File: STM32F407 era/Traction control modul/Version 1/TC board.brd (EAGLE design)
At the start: 79.7 x 100 mm, 70 parts, among them IC1 74HC14D, IC2 lm2575, IC3 74AC08D, IC5 REG1117, IC6 74AC14D, J1 CON1, U1 MAX13052ESA+, U2 MAX232AEWE+, U3 MAX531AESD+, X1 057-006-1

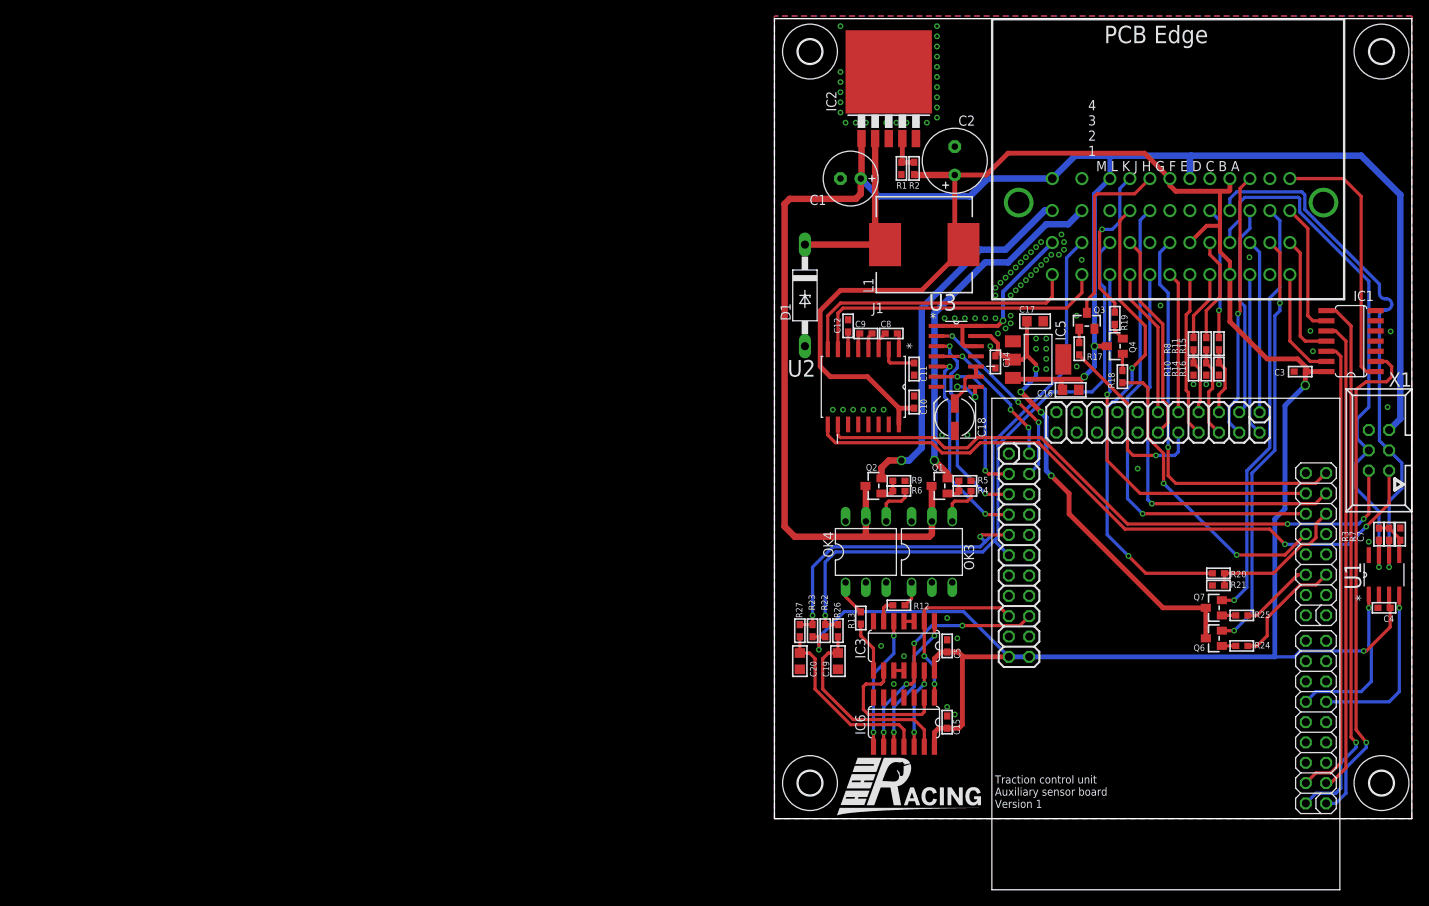
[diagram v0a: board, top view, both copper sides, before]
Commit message: started work on TC V2
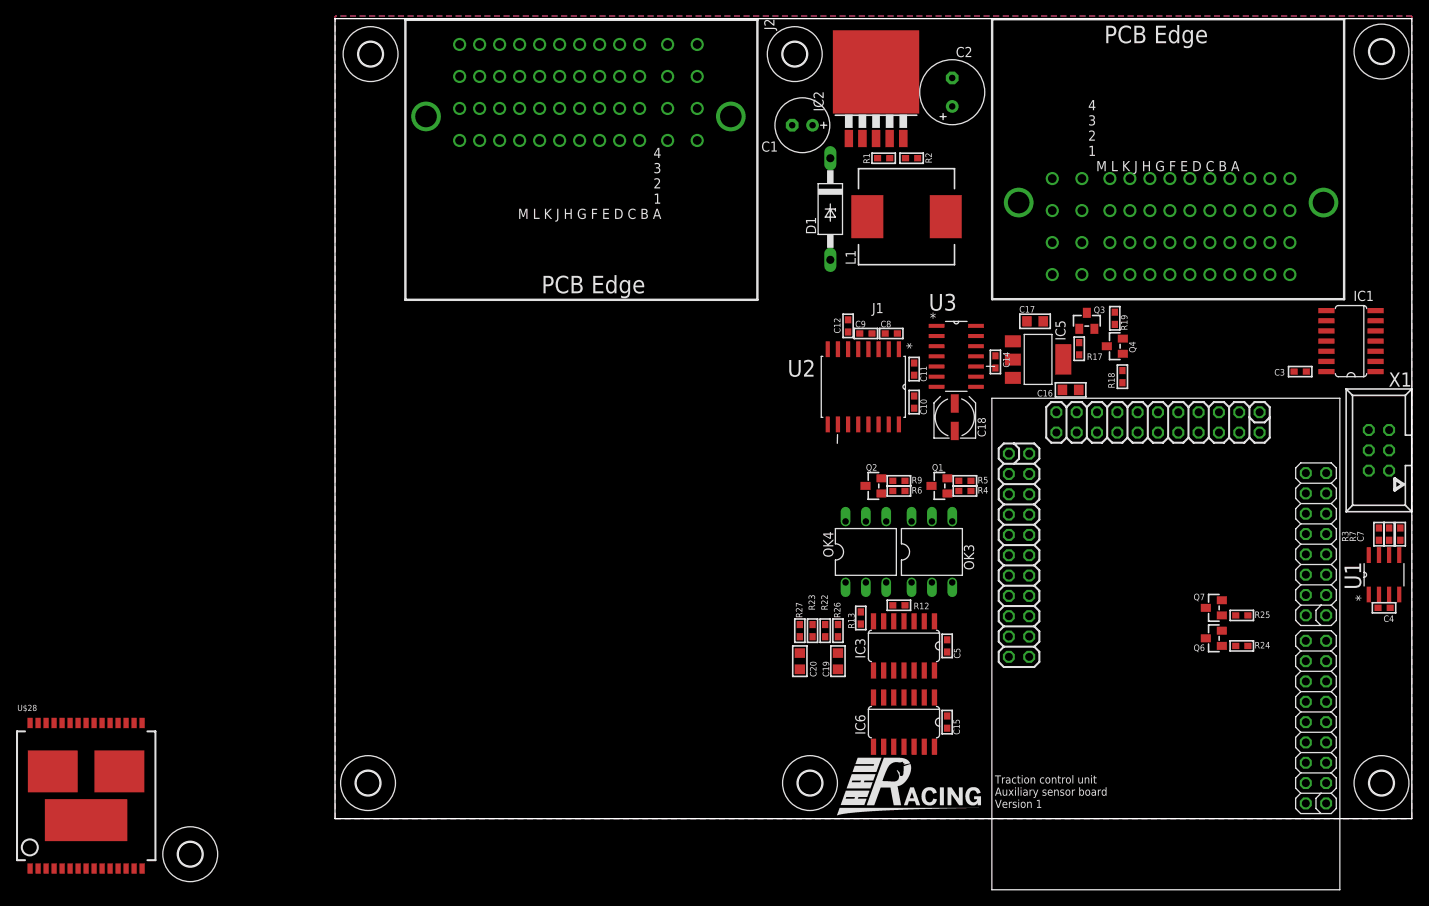
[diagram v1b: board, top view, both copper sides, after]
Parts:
- removed R10, R14, R16, R20: 178, microbuilder:_0603
- removed R11, R15, R21, R8: 604, microbuilder:_0603
- added H5, H6, H7: MOUNT-HOLE3.0, holes:3,0
- added J2: CON1, unicorn_v2:AUTOCONNECTOR
- added U$28: VNH2SP30, SparkFun-PowerIC:VNH2SP30
- moved D1 11.3 mm to (153.0, 92.4)
- moved C1 8.99 mm to (149.5, 102.9)
- moved C2 8.58 mm to (168.3, 107.0)
- moved L1 4.14 mm to (162.6, 91.4)
- moved R1 2.56 mm to (159.7, 98.7), turned to 0 degrees
- moved H2 1.93 mm to (148.6, 111.8)
- moved IC2 1.59 mm to (158.8, 107.0)
- moved R2 1.31 mm to (163.2, 98.7), turned to 180 degrees
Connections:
- net BITE: no longer R15.2
- net BITEO: no longer R15.1, R16.2
- net FUEL-RECIEVE: no longer R21.2
- net FUEL-RECIEVEI: no longer R20.2, R21.1
- net GND: no longer R10.1, R14.1, R16.1, R20.1
- net GSENS: no longer R8.2
- net GSENSO: no longer R10.2, R8.1
- net YAW: no longer R11.2
- net YAWO: no longer R11.1, R14.2
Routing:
- net 3.3V: track 284.1 -> 0.00 mm, vias 3 -> 0
- net 12V: track 235.5 -> 0.00 mm, vias 2 -> 0
- net COMRX: track 84.4 -> 0.00 mm, vias 2 -> 0
- net DIRBSENSE: track 80.9 -> 0.00 mm, vias 1 -> 0
- net COMTX: track 79.3 -> 0.00 mm, vias 2 -> 0
- net DIRASENSE: track 78.7 -> 0.00 mm, vias 2 -> 0
- net CANL: track 69.4 -> 0.00 mm, vias 1 -> 0
- net CANH: track 68.4 -> 0.00 mm, vias 1 -> 0
- net RPM2: track 67.9 -> 0.00 mm, vias 1 -> 0
- net RPM1: track 63.5 -> 0.00 mm, vias 1 -> 0
- net 5.0V: track 62.7 -> 0.00 mm, vias 4 -> 0
- net VTEMP2: track 60.2 -> 0.00 mm, vias 1 -> 0
- net FUEL-RECIEVE: track 59.6 -> 0.00 mm, vias 2 -> 0
- net RPM3: track 59.6 -> 0.00 mm
- net RPM4: track 58.3 -> 0.00 mm
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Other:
- board size 79.7 x 100 mm -> 134.6 x 100 mm

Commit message: Revert "started work on TC V2"
This reverts commit da86986705d51cbc4691d6d7bad1c5aae1ca4806.
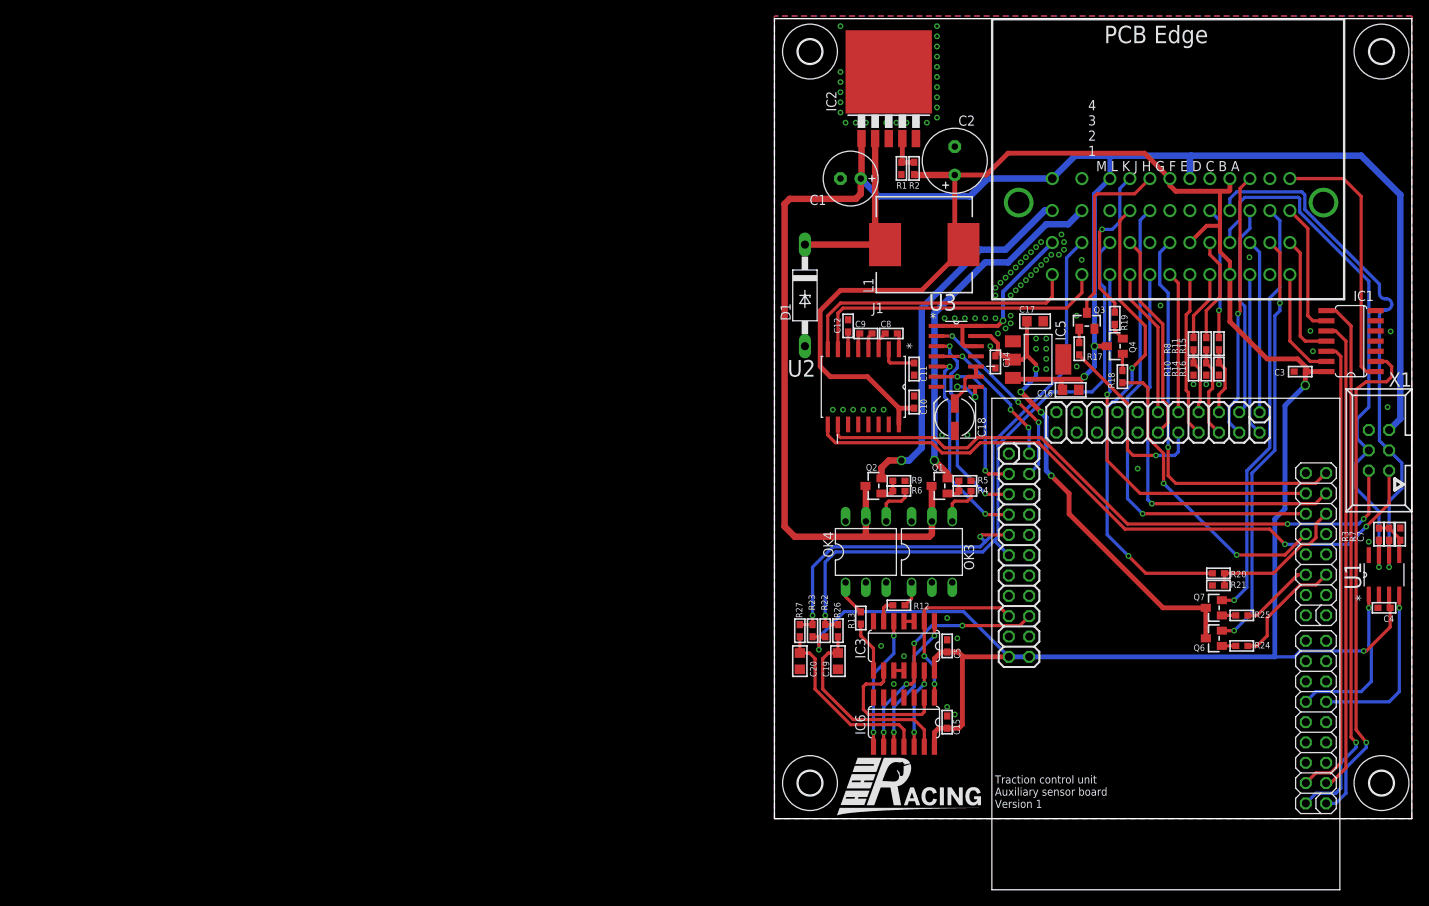
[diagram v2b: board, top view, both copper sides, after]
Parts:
- removed H5, H6, H7: MOUNT-HOLE3.0, holes:3,0
- removed J2: CON1, unicorn_v2:AUTOCONNECTOR
- removed U$28: VNH2SP30, SparkFun-PowerIC:VNH2SP30
- added R10, R14, R16, R20: 178, microbuilder:_0603
- added R11, R15, R21, R8: 604, microbuilder:_0603
- moved D1 11.3 mm to (149.9, 81.6)
- moved C1 8.99 mm to (155.6, 96.2)
- moved C2 8.58 mm to (168.6, 98.4)
- moved L1 4.14 mm to (164.8, 87.9)
- moved R1 2.56 mm to (161.9, 97.5), turned to 90 degrees
- moved H2 1.93 mm to (150.5, 112.1)
- moved IC2 1.59 mm to (160.3, 107.0)
- moved R2 1.31 mm to (163.5, 97.5), turned to 90 degrees
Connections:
- net BITE: now also R15.2
- net BITEO: now also R15.1, R16.2
- net FUEL-RECIEVE: now also R21.2
- net FUEL-RECIEVEI: now also R20.2, R21.1
- net GND: now also R10.1, R14.1, R16.1, R20.1
- net GSENS: now also R8.2
- net GSENSO: now also R10.2, R8.1
- net YAW: now also R11.2
- net YAWO: now also R11.1, R14.2
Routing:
- net 3.3V: track 0.00 -> 284.1 mm, vias 0 -> 3
- net 12V: track 0.00 -> 235.5 mm, vias 0 -> 2
- net COMRX: track 0.00 -> 84.4 mm, vias 0 -> 2
- net DIRBSENSE: track 0.00 -> 80.9 mm, vias 0 -> 1
- net COMTX: track 0.00 -> 79.3 mm, vias 0 -> 2
- net DIRASENSE: track 0.00 -> 78.7 mm, vias 0 -> 2
- net CANL: track 0.00 -> 69.4 mm, vias 0 -> 1
- net CANH: track 0.00 -> 68.4 mm, vias 0 -> 1
- net RPM2: track 0.00 -> 67.9 mm, vias 0 -> 1
- net RPM1: track 0.00 -> 63.5 mm, vias 0 -> 1
- net 5.0V: track 0.00 -> 62.7 mm, vias 0 -> 4
- net VTEMP2: track 0.00 -> 60.2 mm, vias 0 -> 1
- net FUEL-RECIEVE: track 0.00 -> 59.6 mm, vias 0 -> 2
- net RPM3: track 0.00 -> 59.6 mm
- net RPM4: track 0.00 -> 58.3 mm
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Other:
- board size 134.6 x 100 mm -> 79.7 x 100 mm
